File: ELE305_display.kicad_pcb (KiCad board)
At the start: 2 copper layers, 45.7 x 37.5 mm, 5 parts, among them J1 Conn_01x16_Pin, J2 687124182122

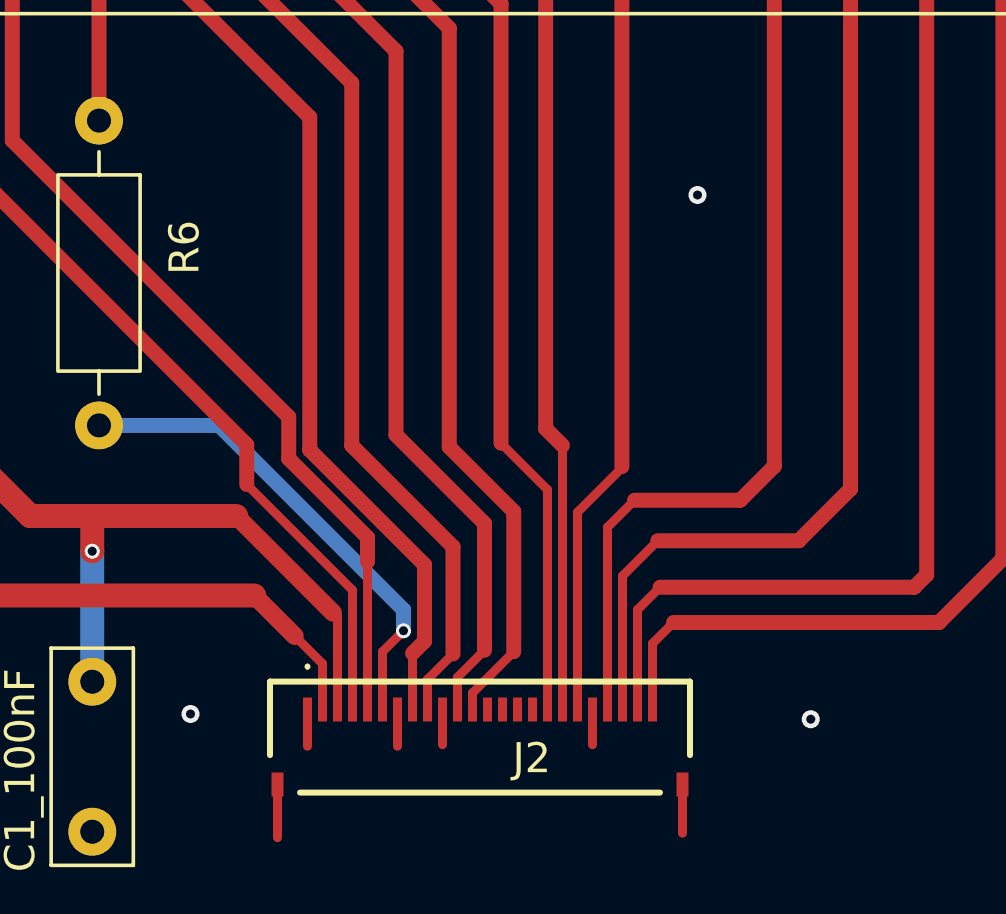
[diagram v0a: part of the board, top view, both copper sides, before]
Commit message: siste endring på pcb-en
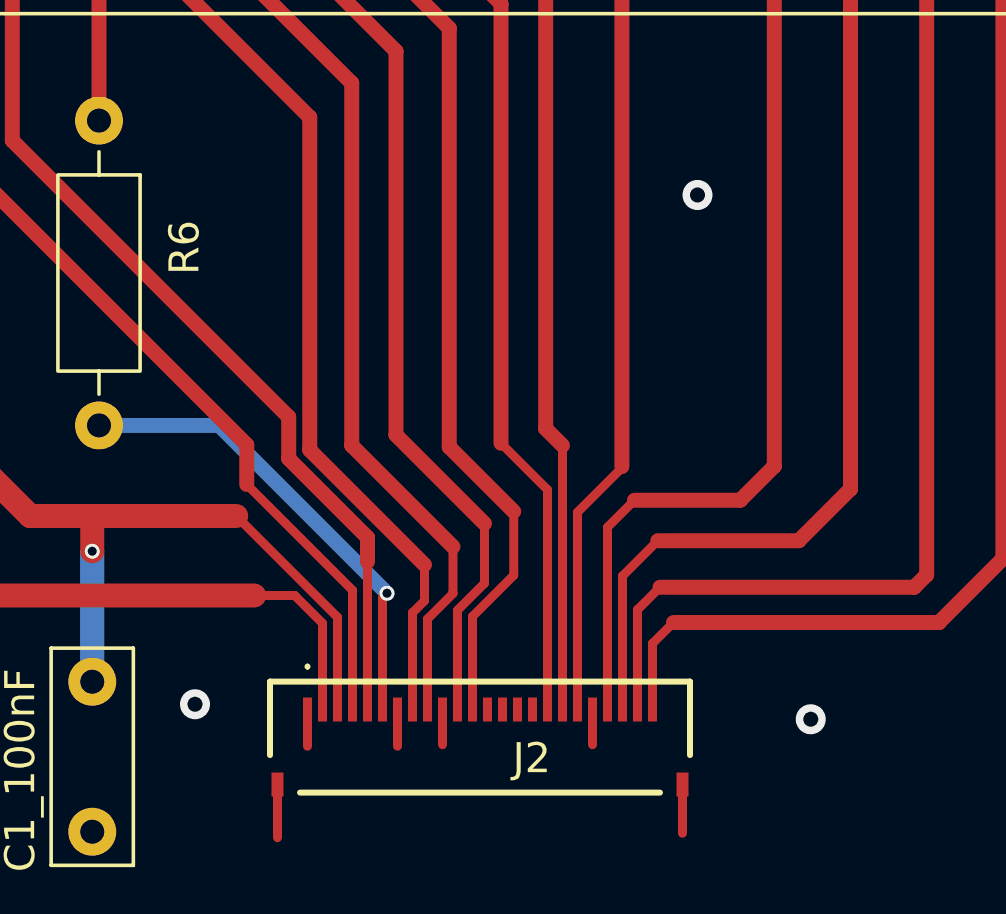
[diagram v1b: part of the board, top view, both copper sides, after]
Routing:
- net Net-(J1-Pin_1): track 69.3 -> 70.1 mm
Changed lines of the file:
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@@
 			(drillshape 0)
 			(scaleselection 1)
-			(outputdirectory "../../mypcb/")
+			(outputdirectory "C:/Users/shafg/Desktop/display_gerber/")
 		)
 	)
@@
 	(via
 		(at 186.775 114.25)
-		(size 0.6)
-		(drill 0.3)
+		(size 1)
+		(drill 0.5)
 		(layers "F.Cu" "B.Cu")
 		(free yes)
@@
 	(via
 		(at 183 96.775)
-		(size 0.6)
-		(drill 0.3)
+		(size 1)
+		(drill 0.5)
 		(layers "F.Cu" "B.Cu")
 		(free yes)
@@
 	)
 	(via
-		(at 166.1 114.075)
-		(size 0.6)
-		(drill 0.3)
+		(at 166.25 113.75)
+		(size 1)
+		(drill 0.5)
 		(layers "F.Cu" "B.Cu")
 		(free yes)
@@
 	)
 	(segment
-		(start 173.2 111.3)
-		(end 172.5 112)
+		(start 172.5 110.2)
+		(end 172.65 110.05)
 		(width 0.3)
 		(layer "F.Cu")
@@
 	)
 	(segment
-		(start 172.5 112)
-		(end 172.5 113.925)
+		(start 172.5 113.925)
+		(end 172.5 110.2)
 		(width 0.3)
 		(layer "F.Cu")
@@
 	)
 	(via
-		(at 173.2 111.3)
+		(at 172.65 110.05)
 		(size 0.5)
 		(drill 0.3)
@@
 	)
 	(segment
-		(start 173.2 111.3)
-		(end 173.2 110.6)
-		(width 0.5)
-		(layer "B.Cu")
-		(net 3)
-	)
-	(segment
-		(start 173.2 110.6)
+		(start 172.65 110.05)
 		(end 167.055 104.455)
 		(width 0.5)
@@
 	)
 	(segment
-		(start 170.849 110.699)
-		(end 167.625 107.475)
-		(width 0.6)
-		(layer "F.Cu")
-		(net 7)
-	)
-	(segment
-		(start 170.5 113.925)
-		(end 170.5 112.4)
-		(width 0.3)
-		(layer "F.Cu")
-		(net 7)
-	)
-	(segment
 		(start 156.825 113)
 		(end 156.825 108.975)
@@
 	)
 	(segment
+		(start 171 110.85)
+		(end 167.625 107.475)
+		(width 0.3)
+		(layer "F.Cu")
+		(net 7)
+	)
+	(segment
 		(start 155.08 107.23)
 		(end 155.08 103.525)
@@
 	)
 	(segment
-		(start 170.5 112.4)
-		(end 169.575 111.475)
-		(width 0.3)
-		(layer "F.Cu")
-		(net 7)
-	)
-	(segment
-		(start 171 110.85)
-		(end 170.849 110.699)
-		(width 0.3)
-		(layer "F.Cu")
-		(net 7)
-	)
-	(segment
 		(start 162.825 107.475)
 		(end 162.825 108.65)
@@
 	)
 	(segment
+		(start 170.5 111.05)
+		(end 169.575 110.125)
+		(width 0.3)
+		(layer "F.Cu")
+		(net 7)
+	)
+	(segment
 		(start 155.08 101.8)
 		(end 155.08 89.35)
@@
 	)
 	(segment
-		(start 168.225 110.125)
-		(end 169.575 111.475)
-		(width 0.6)
-		(layer "F.Cu")
-		(net 7)
-	)
-	(segment
 		(start 167.625 107.475)
 		(end 162.825 107.475)
@@
 	)
 	(segment
+		(start 170.5 113.925)
+		(end 170.5 111.05)
+		(width 0.3)
+		(layer "F.Cu")
+		(net 7)
+	)
+	(segment
 		(start 157.975 110.125)
 		(end 156.825 108.975)
 		(width 0.8)
+		(layer "F.Cu")
+		(net 7)
+	)
+	(segment
+		(start 169.575 110.125)
+		(end 168.225 110.125)
+		(width 0.3)
 		(layer "F.Cu")
 		(net 7)
@@
 	)
 	(segment
-		(start 174 112.925)
-		(end 174.85 112.075)
-		(width 0.3)
-		(layer "F.Cu")
-		(net 10)
-	)
-	(segment
 		(start 171.475 105.125)
 		(end 171.475 93.045)
@@
 	)
 	(segment
-		(start 174.85 112.075)
+		(start 174.85 110.05796)
 		(end 174.85 108.5)
-		(width 0.5)
+		(width 0.3)
 		(layer "F.Cu")
 		(net 10)
 	)
 	(segment
+		(start 174 110.90796)
+		(end 174.85 110.05796)
+		(width 0.3)
+		(layer "F.Cu")
+		(net 10)
+	)
+	(segment
 		(start 174 113.925)
-		(end 174 112.925)
+		(end 174 110.90796)
 		(width 0.3)
 		(layer "F.Cu")
@@
 	)
 	(segment
-		(start 173.5 113.925)
-		(end 173.5 112.05)
+		(start 173.5 110.7)
+		(end 173.9 110.3)
+		(width 0.3)
+		(layer "F.Cu")
+		(net 14)
+	)
+	(segment
+		(start 173.9 110.3)
+		(end 173.9 109.1)
 		(width 0.3)
 		(layer "F.Cu")
@@
 	)
 	(segment
-		(start 173.5 112.05)
-		(end 173.9 111.65)
-		(width 0.5)
-		(layer "F.Cu")
-		(net 14)
-	)
-	(segment
-		(start 173.9 111.65)
-		(end 173.9 109.1)
-		(width 0.5)
+		(start 173.5 113.925)
+		(end 173.5 110.7)
+		(width 0.3)
 		(layer "F.Cu")
 		(net 14)
@@
 	)
 	(segment
+		(start 171.5 111.425)
+		(end 171.5 109.95)
+		(width 0.3)
+		(layer "F.Cu")
+		(net 17)
+	)
+	(segment
 		(start 171.5 113.925)
-		(end 171.5 109.95)
+		(end 171.5 111.425)
 		(width 0.3)
 		(layer "F.Cu")
@@
 	(segment
 		(start 175.5 113.925)
-		(end 175.5 113.375)
+		(end 175.5 110.825)
 		(width 0.3)
 		(layer "F.Cu")
@@
 	)
 	(segment
-		(start 176.875 112)
-		(end 176.875 107.325)
-		(width 0.5)
+		(start 175.5 110.825)
+		(end 176.875 109.45)
+		(width 0.3)
 		(layer "F.Cu")
 		(net 18)
@@
 	)
 	(segment
-		(start 175.5 113.375)
-		(end 176.875 112)
+		(start 176.875 109.45)
+		(end 176.875 107.325)
 		(width 0.3)
 		(layer "F.Cu")
@@
 	(segment
 		(start 175 113.925)
-		(end 175 112.85)
+		(end 175 111.03352)
 		(width 0.3)
 		(layer "F.Cu")
@@
 	)
 	(segment
-		(start 175.9 111.95)
+		(start 174.999 110.61748)
+		(end 175.9 109.71648)
+		(width 0.3)
+		(layer "F.Cu")
+		(net 20)
+	)
+	(segment
+		(start 175.9 109.71648)
 		(end 175.9 107.725)
-		(width 0.5)
-		(layer "F.Cu")
-		(net 20)
-	)
-	(segment
-		(start 175 112.85)
-		(end 175.9 111.95)
 		(width 0.3)
 		(layer "F.Cu")
@@
 		(layer "F.Cu")
 		(net 20)
+	)
+	(segment
+		(start 175 111.03352)
+		(end 174.999 111.03252)
+		(width 0.3)
+		(layer "F.Cu")
+		(net 20)
+	)
+	(segment
+		(start 174.999 111.03252)
+		(end 174.999 110.61748)
+		(width 0.3)
+		(layer "F.Cu")
+		(net 20)
